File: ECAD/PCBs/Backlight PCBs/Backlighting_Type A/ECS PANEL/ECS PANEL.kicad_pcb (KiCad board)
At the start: 2 copper layers, 133.6 x 93 mm, 160 parts, among them J1 Mini-Fit Jr. 2x02, J2 Mini-Fit Jr. 2x02

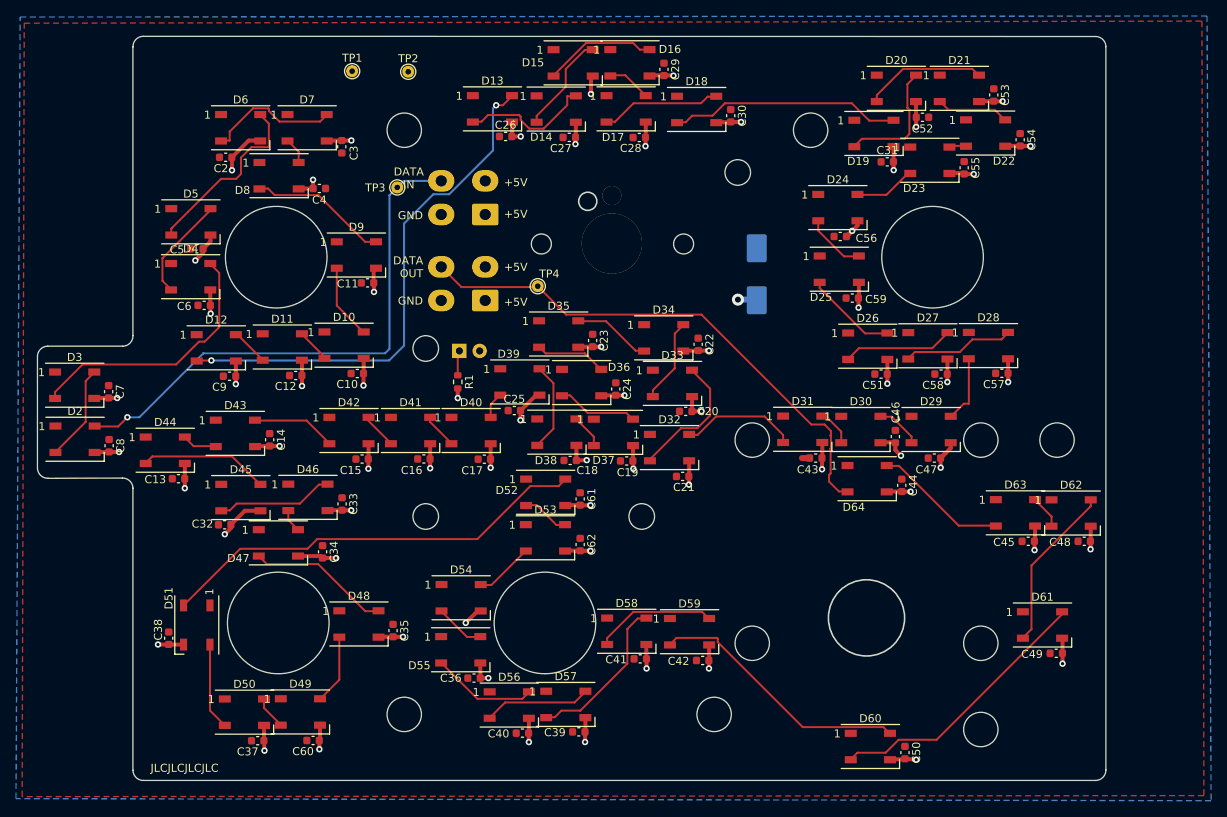
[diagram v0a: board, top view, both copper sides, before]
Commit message: Revert "Merge branch 'jrsteensen:v1.0.0-beta1' into v1.0.0-beta1"
This reverts commit 46e82843c31f9b05e538ac2419630b7d41e62aa3, reversing
changes made to 65c8b9758aa9b916aef14988de7149d3308c9d9a.
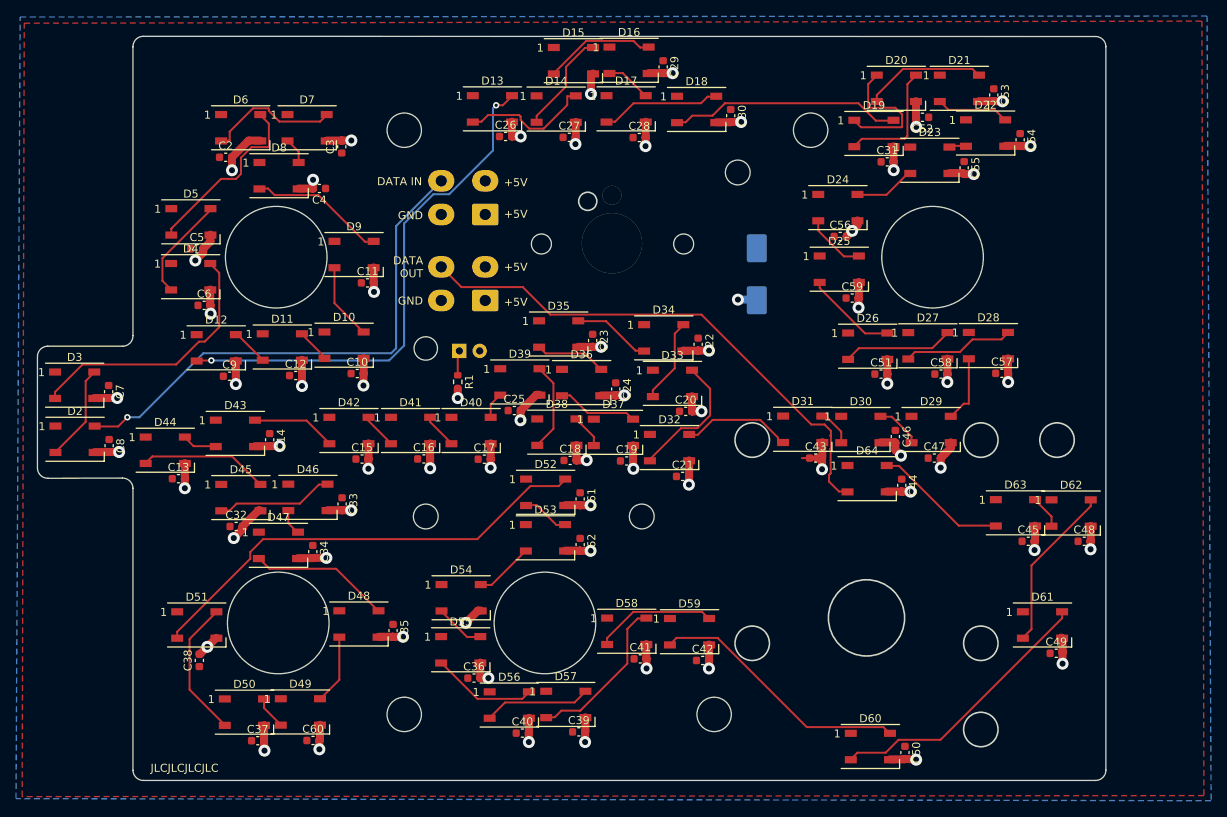
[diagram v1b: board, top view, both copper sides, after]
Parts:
- removed MH1, MH10, MH2, MH3, MH4, MH5, MH6, MH7, MH8, MH9: 6x32 / 4mm, OH_Footprints:MountingHole_6-32_PHS
- removed MH11, MH12, MH13, MH14: M3 / 3.2mm, OH_Footprints:MountingHole_3.2mm_M3_DIN965
- removed MH15, MH16: 2.5mm, OH_Footprints:MountingHole_2.5mm
- removed MH17, MH18: Switch_NKK SxAL, OH_Footprints:SxAL_Toggle_13x13mm
- removed MH19, MH20: Switch_631H, OH_Footprints:631HX_Toggle_13mm_x_13mm
- removed MH21: Pot_B10K, OH_Footprints:BR10K_Pot_11mm_x_11mm
- removed TP1, TP2, TP3, TP4: TestPoint, OH_Footprints:TestPoint_THTPad_D1.5mm_Drill0.7mm
- added 1: SxAL_Toggle_13x13mm, OH_Footprints:SxAL_Toggle_13x13mm, F.Cu at (105.5, 71.9)
- added 3: SxAL_Toggle_13x13mm, OH_Footprints:SxAL_Toggle_13x13mm, F.Cu at (187.6, 71.9)
- added 5: 631H_Toggle_13mm_x_13mm, OH_Footprints:631H_Toggle_13mm_x_13mm, F.Cu at (105.8, 117.6)
- added REF**: 631H_Toggle_13mm_x_13mm, OH_Footprints:631H_Toggle_13mm_x_13mm, F.Cu at (139.1, 117.6)
- added REF**: BR10K_Pot_11mm_x_11mm, OH_Footprints:BR10K_Pot_11mm_x_11mm, F.Cu at (147.5, 70.1)
- added REF**: OH_Panel_Fastner_Keepout, OH_Footprints:OH_Panel_6-32_PHS, F.Cu at (121.5, 56.0)
- added REF**: OH_Panel_Fastner_Keepout, OH_Footprints:OH_Panel_6-32_PHS, F.Cu at (172.3, 56.0)
- added REF**: OH_Panel_Fastner_Keepout, OH_Footprints:OH_Panel_6-32_PHS, F.Cu at (160.3, 129.0)
- added REF**: OH_Panel_Fastner_Keepout, OH_Footprints:OH_Panel_6-32_PHS, F.Cu at (121.5, 129.0)
- added REF**: MountingHole, OH_Footprints:MountingHole_2.5mm, F.Cu at (138.7, 70.2)
- added REF**: MountingHole, OH_Footprints:MountingHole_2.5mm, F.Cu at (156.4, 70.2)
- C1: value 1000uF -> C_Polarized
- C10, C11, C12, C13, C14, C15, C16, C17, C18, C19, C2, C20, C21, C22, C23, C24, C25, C26, C27, C28, C29, C3, C30, C31, C32, C33, C34, C35, C36, C37, C38, C39, C4, C40, C41, C42, C43, C44, C45, C46, C47, C48, C49, C5, C50, C51, C52, C53, C54, C55, C56, C57, C58, C59, C6, C60, C61, C62, C7, C8, C9: value 0.1uF -> C
- D1: value Green -> LED
- G*** (x2): moved to F.Cu
- G***: footprint OH_Footprints:631H2_Toggle_Silkscreen -> OH_Footprints:631H_Toggle_Silkscreen; moved to F.Cu
- G***: footprint OH_Footprints:631H3_Toggle_Silkscreen -> OH_Footprints:631H_Toggle_Silkscreen; moved to F.Cu
- G***: renamed from LOGO2; footprint OH_Footprints:LOGO_CC-BY-NC-SA_Half_Small -> OH_Footprints:CC-BY-NC-SA-Small
- G***: renamed from LOGO1; footprint OH_Footprints:LOGO_OH_Text_Large -> OH_Footprints:OH_LOGO_37.7mm_5.9mm
- J1, J2: value Mini-Fit Jr. 2x02 -> Conn_01x04_Female
- R1: value 470 -> R
- moved G*** 8.96 mm to (139.4, 93.7)
- moved C38 4.73 mm to (95.9, 122.3), turned to 90 degrees
- moved C32 1.46 mm to (100.5, 105.5)
- moved G*** 1.42 mm to (94.9, 72.0), turned to 0 degrees
- moved G*** 1.29 mm to (177.4, 72.5), turned to 0 degrees
- moved C34 1.22 mm to (110.1, 108.7)
- moved G*** 1.03 mm to (127.7, 118.3), turned to 0 degrees
- moved G*** 1.02 mm to (94.3, 118.0), turned to 0 degrees
- moved D16 0.33 mm to (149.6, 47.3)
- moved C29 0.33 mm to (153.9, 48.1)
- moved D47 0.31 mm to (105.8, 107.9)
- moved D9 0.30 mm to (115.2, 71.6)
- moved D15 0.27 mm to (142.7, 47.3)
- turned D51 to 0 degrees
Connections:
- net +5V renamed /LED+5V
- net /DATA1 renamed Net-(D14-Pad2)
- net /DATA2 renamed Net-(D27-Pad2)
- net /DATA3 renamed Net-(D40-Pad2)
- net /DATA4 renamed Net-(D53-Pad2)
- net DATA IN renamed /DATAIN
- net DATA OUT renamed /DATAOUT
- net GND renamed /LEDGND
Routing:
- net /LED+5V: track 3.22 -> 20.2 mm
- net Net-(D50-Pad2): track 10.9 -> 17.3 mm
- net Net-(D51-Pad2): track 54.2 -> 57.6 mm
- net /DATAIN: track 67.3 -> 65.0 mm
- net /DATAOUT: track 66.6 -> 68.3 mm
- net /LEDGND: track 203.6 -> 205.3 mm
- net Net-(D31-Pad2): track 14.6 -> 13.4 mm
- net Net-(D30-Pad2): track 4.01 -> 5.12 mm
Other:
- outline, holes or cut-outs redrawn
- board text added: "3"
- board text added: "BLEED AIR"
- board text added: "ECS PANEL Revision: 3 www.openhornet.com"
- board text added: "IN"
- board text added: "Switch PCB H1"
- board text added: "Switch PCB H2"
- board text added: "Switch PCB H3"
- board text added: "Switch PCB H4"
- board text added: "THRU"
- board text added: "⌀3MM"
- board text added: "⌀4MM"
- board text removed: "0.2000 mm"
- board text removed: "0.2000 mm / 0.1270 mm"
- board text removed: "1.6000 mm"
- board text removed: "133.5532 mm x 93.0148 mm"
- board text removed: "BOARD CHARACTERISTICS"
- board text removed: "Board Thickness:"
- board text removed: "Board overall dimensions:"
- board text removed: "Castellated pads:"
- board text removed: "Copper Finish:"
- board text removed: "Copper Layer Count:"
- board text removed: "ECS PANEL REV: 4 WWW.OPENHORNET.COM"
- board text removed: "Edge card connectors:"
- board text removed: "Impedance Control:"
- board text removed: "Min hole diameter:"
- board text removed: "Min track/spacing:"
- board text removed: "No"
- board text removed: "None"
- board text removed: "Plated Board Edge:"
